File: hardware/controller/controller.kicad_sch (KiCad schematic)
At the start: 4 parts, among them U1 ZX-PM2.54-1-16PY, U2 ZX-PM2.54-1-16PY, U3 ZX-PM2.54-1-16PY, U4 ZX-PM2.54-1-16PY

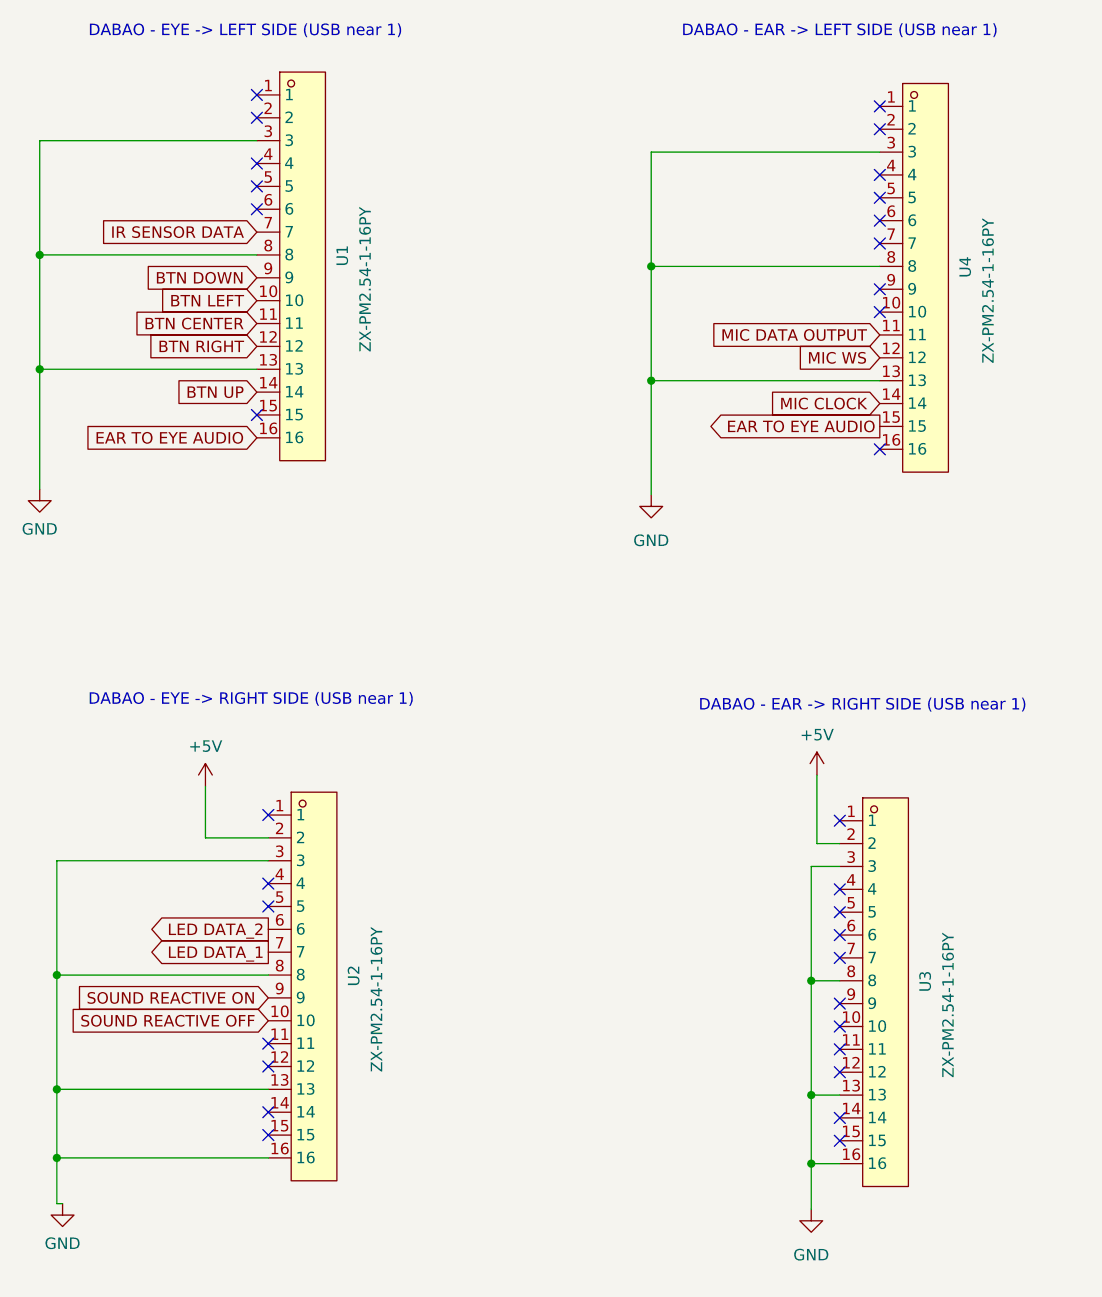
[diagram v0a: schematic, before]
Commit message: controller layout updates
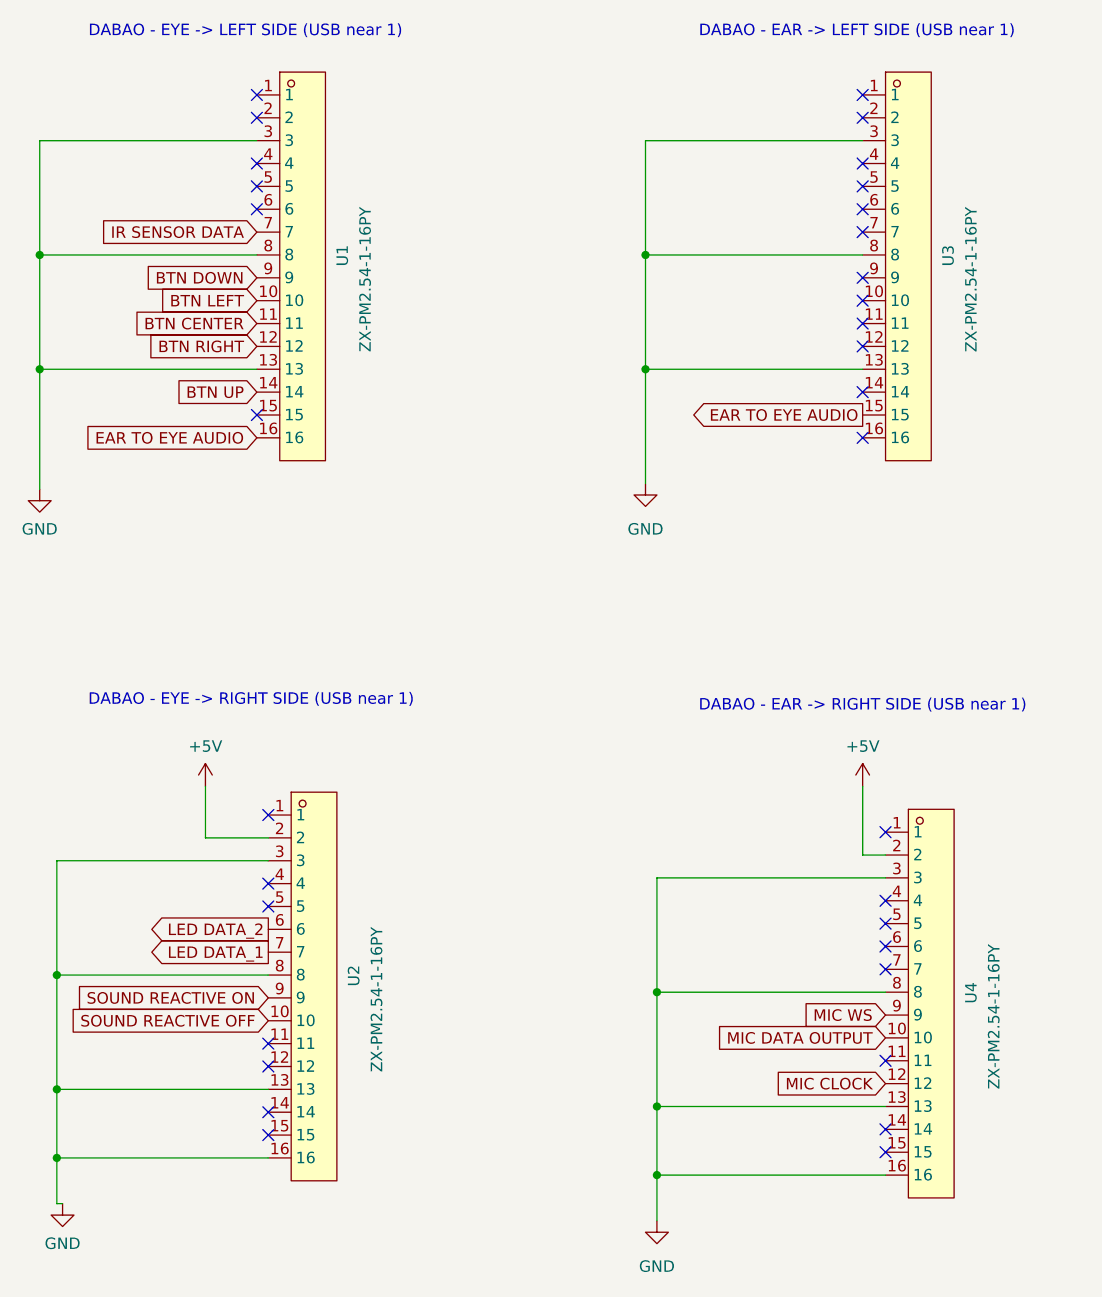
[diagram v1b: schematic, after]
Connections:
- net +5V: now also U4.2; no longer U3.2
- net EAR TO EYE AUDIO: now also U3.15; no longer U4.15
- net GND: now also U4.16; no longer U3.16
- net MIC CLOCK: now also U4.12; no longer U4.14
- net MIC DATA OUTPUT: now also U4.10; no longer U4.11
- net MIC WS: now also U4.9; no longer U4.12
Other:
- moved on the sheet: U3, U4
